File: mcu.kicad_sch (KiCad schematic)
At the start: 15 parts, among them U3 STM32L431CBT6

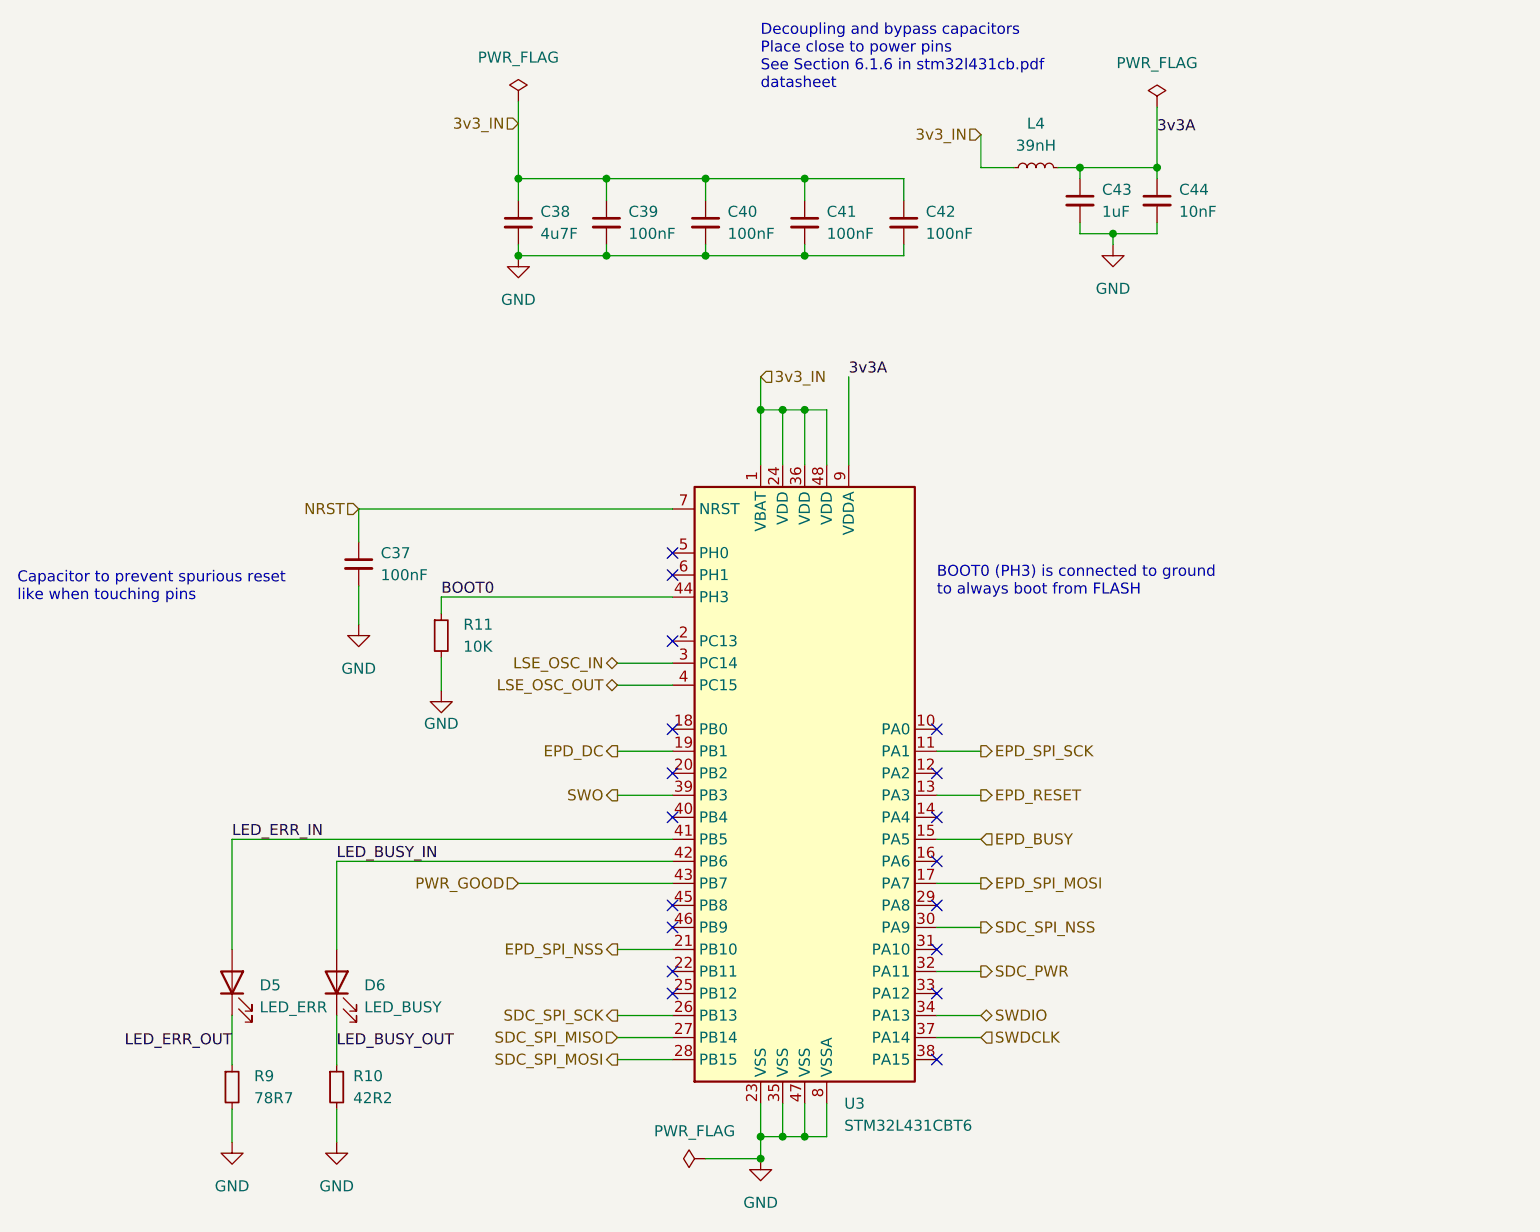
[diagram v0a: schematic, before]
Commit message: Revision 1 of the board that was manufactured
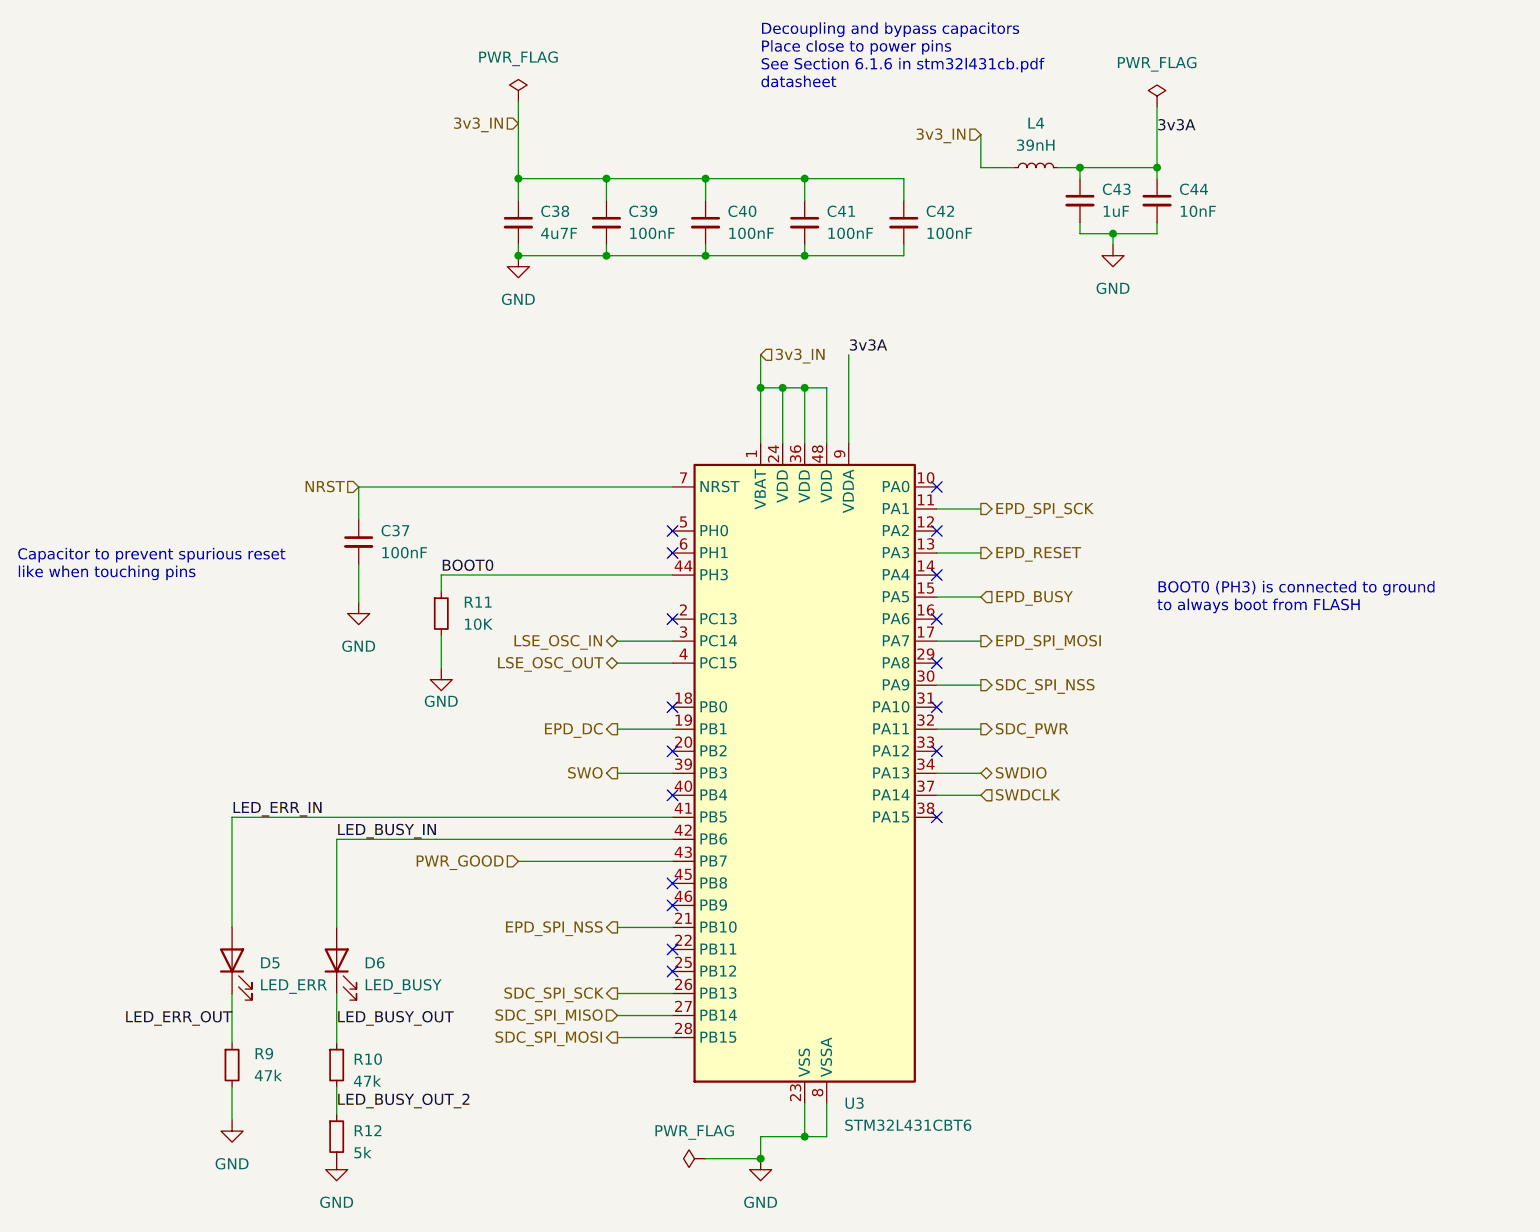
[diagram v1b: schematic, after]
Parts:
- added R12: 5k, Resistor_SMD:R_1206_3216Metric, symbol Device:R_Small
- C37, C39, C40, C41, C42: LCSC (none) -> C14663
- C38: LCSC (none) -> C19666
- C43: LCSC (none) -> C15849
- C44: LCSC (none) -> C57112
- L4: LCSC (none) -> C440213
- R10: value 42R2 -> 47k; LCSC (none) -> C230465
- R11: LCSC (none) -> C510098
- R9: value 78R7 -> 47k; LCSC (none) -> C230465
- U3: LCSC (none) -> C277951
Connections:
- net GND: now also R12.2; no longer R10.2
- new net LED_BUSY_OUT_2: R10.2, R12.1
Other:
- moved on the sheet: C37, D5, D6, R10, R11, R9
